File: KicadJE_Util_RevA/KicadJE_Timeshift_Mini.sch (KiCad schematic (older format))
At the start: 51 parts

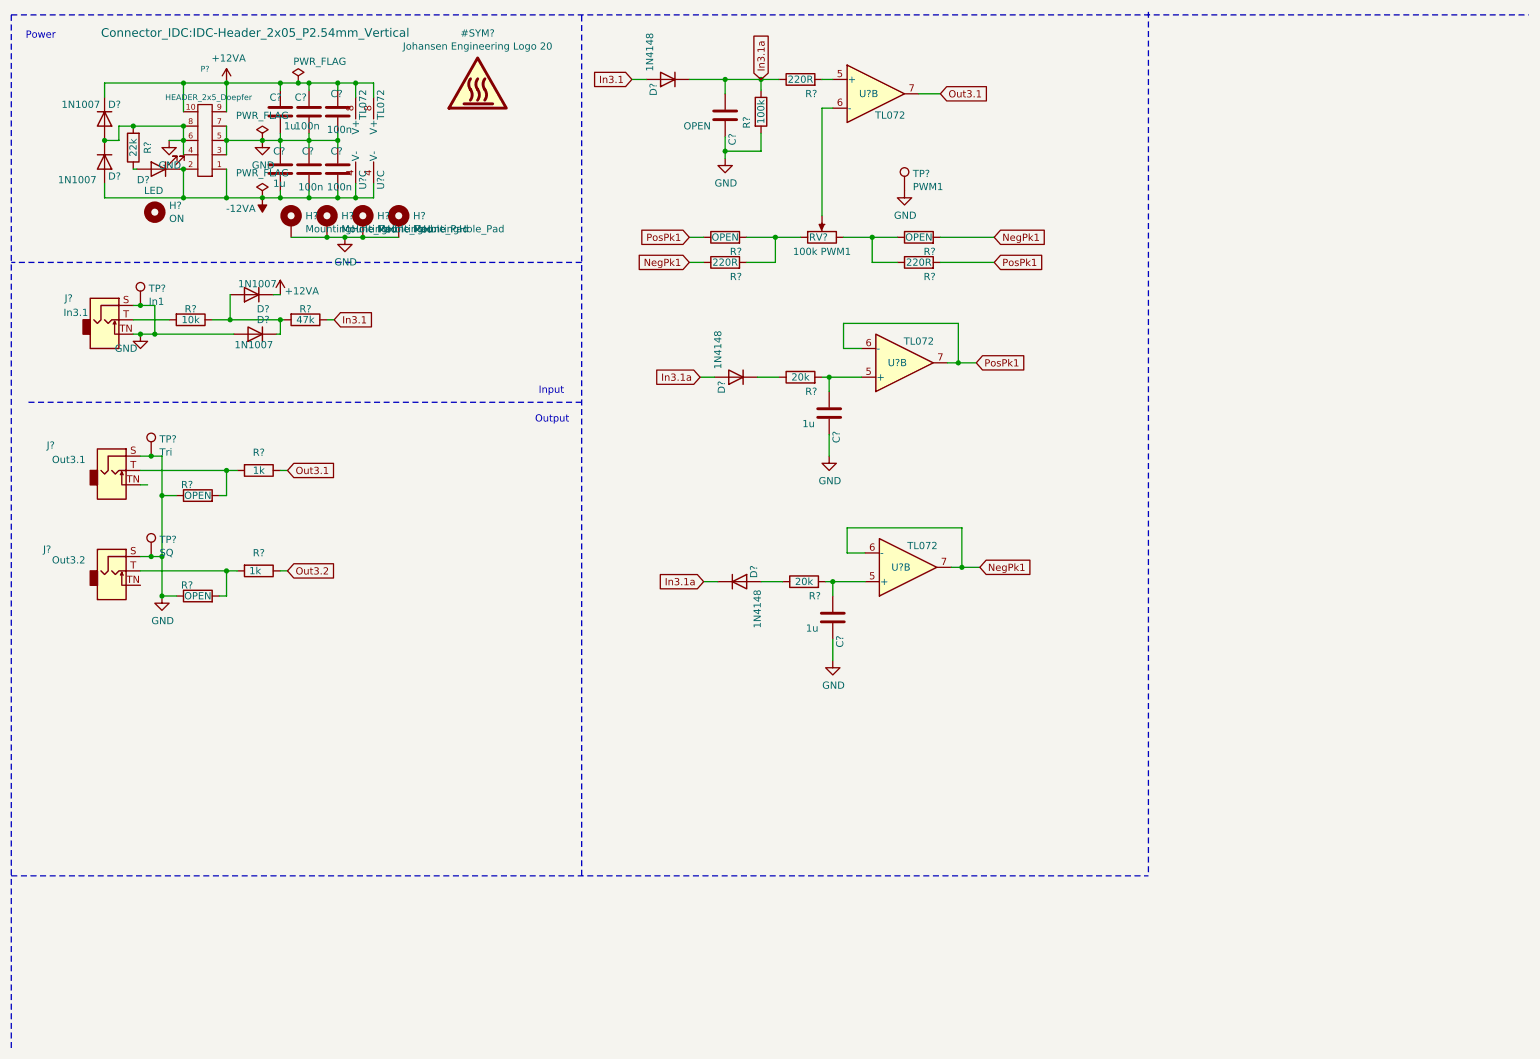
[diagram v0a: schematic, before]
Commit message: Update KicadJE_Timeshift_Mini.sch
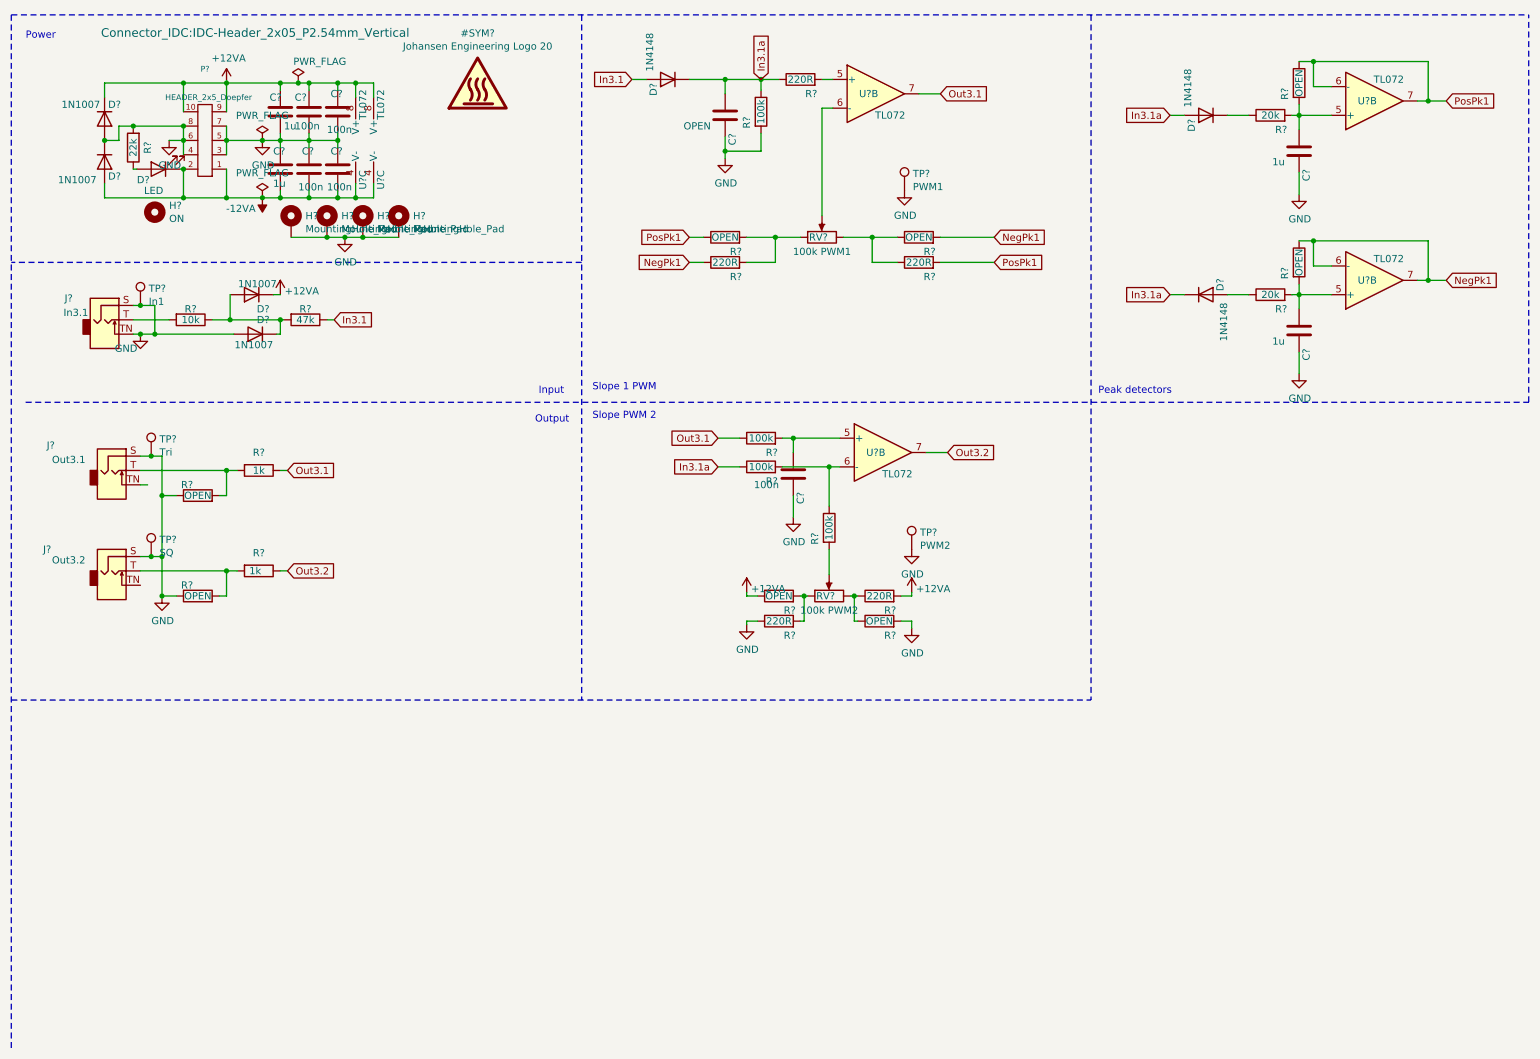
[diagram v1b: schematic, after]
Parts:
- added C?: 100n, Capacitor_SMD:C_0805_2012Metric_Pad1.15x1.40mm_HandSolder, symbol Device:C
- added R? (x4): OPEN, Resistor_SMD:R_0805_2012Metric_Pad1.15x1.40mm_HandSolder, symbol Device:R
- added R? (x2): 220R, Resistor_SMD:R_0805_2012Metric_Pad1.15x1.40mm_HandSolder, symbol Device:R
- added R? (x3): 100k, Resistor_SMD:R_0805_2012Metric_Pad1.15x1.40mm_HandSolder, symbol Device:R
- added RV?: 100k PWM2, AJ-Dropbox-Kicad:Potentiometer_China_RK09_Single_Vertical_AJ, symbol Envelope-cache-2018-08-04-13-00-04:POT
- added TP?: PWM2, AJ:Pot_6m3_scale1, symbol Connector:TestPoint
- added U?: TL072, AJ-Dropbox-Kicad:AJ_SO-8_5.3x6.2mm_P1.27mm, symbol Amplifier_Operational:TL072
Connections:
- net +12VA: now also R?.1, R?.2
- net GND: now also C?.1, R?.1, R?.2, TP?.1
- net In3.1a: now also R?.1
- net NegPk1: now also R?.1
- net Out3.1: now also R?.1
- net Out3.2: now also U?.7
- net PosPk1: now also R?.1
- net at C?.2, R?.2, U?.5 (+): now also R?.2 (x2)
- new net: C?.2, R?.2, U?.5 (+)
- new net: R?.1, R?.2, U?.6 (-)
- new net: R?.2, R?.2, RV?.1
- new net: R?.2, RV?.2
- new net: R?.1, R?.1, RV?.3
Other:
- note added: "Peak detectors"
- note added: "Slope 1 PWM"
- note added: "Slope PWM 2"
- moved on the sheet: C?, D?, R?, U?B
